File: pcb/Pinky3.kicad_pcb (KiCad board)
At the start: 2 copper layers, 137 x 100.9 mm, 67 parts, among them J1 MJ-4PP-9, P1 i2c-pin, P2 i2c-pin, SW1 RESET_SW, SW10 SW_PUSH, SW11 SW_PUSH, SW12 SW_PUSH, SW13 SW_PUSH, SW14 SW_PUSH, SW15 SW_PUSH, SW16 SW_PUSH, SW17 SW_PUSH, SW18 SW_PUSH, SW19 SW_PUSH, SW2 SW_PUSH, SW20 SW_PUSH, SW21 SW_PUSH, SW22 SW_PUSH, SW23 SW_PUSH, SW24 SW_PUSH, SW25 SW_PUSH, SW26 SW_PUSH, SW3 SW_PUSH, SW4 SW_PUSH, SW5 SW_PUSH, SW6 SW_PUSH, SW7 SW_PUSH, SW8 SW_PUSH, SW9 SW_PUSH, U1 ProMicro

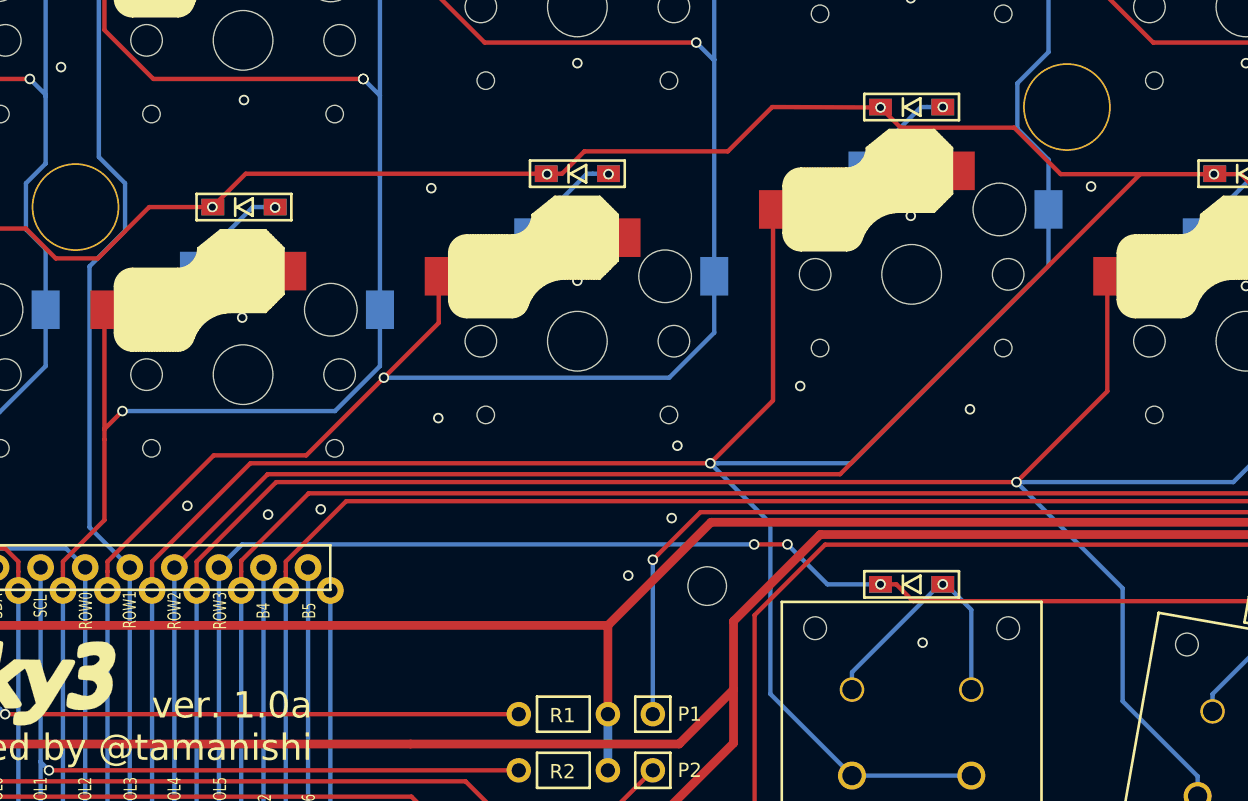
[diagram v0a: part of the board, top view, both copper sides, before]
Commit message: tweak row2
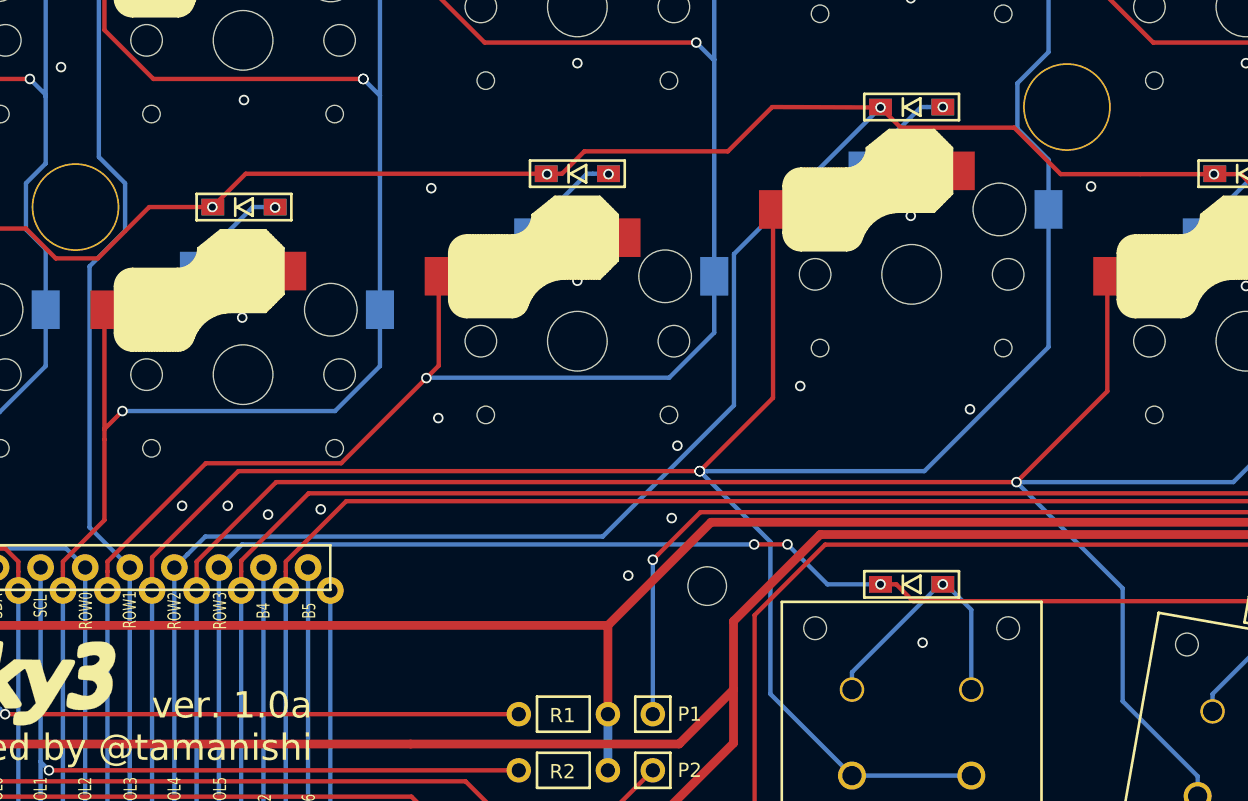
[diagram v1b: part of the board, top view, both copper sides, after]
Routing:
- net row2: track 200.4 -> 192.3 mm
- net col3: track 201.4 -> 204.8 mm, vias 4 -> 5
- net col2: track 145.2 -> 144.2 mm
- net GND: vias 56 -> 57
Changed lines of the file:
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@@
     (thickness 1.6)
     (drawings 29)
-    (tracks 910)
+    (tracks 912)
     (zones 0)
     (modules 67)
@@
   (segment (start 154.85 103.3) (end 156.325 103.3) (width 0.25) (layer F.Cu) (net 7))
   (segment (start 152.32499 100.77499) (end 154.85 103.3) (width 0.25) (layer F.Cu) (net 7))
-  (segment (start 113.876999 102.023001) (end 120.175 95.725) (width 0.25) (layer F.Cu) (net 7))
-  (segment (start 113.875001 102.023001) (end 113.876999 102.023001) (width 0.25) (layer F.Cu) (net 7))
-  (segment (start 103.073012 112.82499) (end 113.875001 102.023001) (width 0.25) (layer F.Cu) (net 7))
-  (segment (start 70.45061 112.82499) (end 103.073012 112.82499) (width 0.25) (layer F.Cu) (net 7))
-  (segment (start 65.132 118.1436) (end 70.45061 112.82499) (width 0.25) (layer F.Cu) (net 7))
   (segment (start 120.175 95.725) (end 115.643998 95.725) (width 0.25) (layer F.Cu) (net 7))
   (segment (start 120.175 95.725) (end 124.375 95.725) (width 0.25) (layer F.Cu) (net 7))
+  (segment (start 66.90061 116.37499) (end 65.893999 117.381601) (width 0.25) (layer B.Cu) (net 7))
+  (segment (start 65.893999 117.381601) (end 65.132 118.1436) (width 0.25) (layer B.Cu) (net 7))
+  (segment (start 89.550012 116.37499) (end 66.90061 116.37499) (width 0.25) (layer B.Cu) (net 7))
+  (segment (start 97.025001 108.900001) (end 89.550012 116.37499) (width 0.25) (layer B.Cu) (net 7))
+  (segment (start 97.025001 100.274999) (end 97.025001 108.900001) (width 0.25) (layer B.Cu) (net 7))
+  (segment (start 105.375 91.925) (end 97.025001 100.274999) (width 0.25) (layer B.Cu) (net 7))
   (segment (start 89.7 74.8) (end 89.875 74.8) (width 0.25) (layer B.Cu) (net 8))
   (segment (start 85.3 70.4) (end 89.7 74.8) (width 0.25) (layer B.Cu) (net 8))
@@
   (via (at 144.575 113.525) (size 0.6) (drill 0.4) (layers F.Cu B.Cu) (net 30))
   (via (at 70.475 115.125) (size 0.6) (drill 0.4) (layers F.Cu B.Cu) (net 30))
-  (via (at 65.875 114.625) (size 0.6) (drill 0.4) (layers F.Cu B.Cu) (net 30))
   (via (at 163.175 111.625) (size 0.6) (drill 0.4) (layers F.Cu B.Cu) (net 30))
+  (via (at 65.575 114.625) (size 0.6) (drill 0.4) (layers F.Cu B.Cu) (net 30))
+  (via (at 68.175 114.625) (size 0.6) (drill 0.4) (layers F.Cu B.Cu) (net 30))
   (segment (start 48.622 133.024838) (end 48.622 134.69) (width 0.25) (layer B.Cu) (net 31) (status 20))
   (segment (start 47.352 131.754838) (end 48.622 133.024838) (width 0.25) (layer B.Cu) (net 31))
@@
   (segment (start 95.85 89.2) (end 95.9 89.2) (width 0.25) (layer B.Cu) (net 38))
   (segment (start 95.9 70.4) (end 95.9 89.2) (width 0.25) (layer B.Cu) (net 38))
-  (segment (start 80.2 101.545) (end 80.2 104.198998) (width 0.25) (layer F.Cu) (net 38))
-  (segment (start 95.9 104.758002) (end 93.333002 107.325) (width 0.25) (layer B.Cu) (net 38))
-  (segment (start 95.9 101.545) (end 95.9 104.758002) (width 0.25) (layer B.Cu) (net 38))
-  (via (at 77.074499 107.324499) (size 0.6) (drill 0.4) (layers F.Cu B.Cu) (net 38))
-  (segment (start 77.075 107.325) (end 77.074499 107.324499) (width 0.25) (layer B.Cu) (net 38))
-  (segment (start 93.333002 107.325) (end 77.075 107.325) (width 0.25) (layer B.Cu) (net 38))
-  (segment (start 80.2 104.198998) (end 77.074499 107.324499) (width 0.25) (layer F.Cu) (net 38))
   (segment (start 61.322 119.45) (end 61.322 132.078) (width 0.25) (layer B.Cu) (net 38))
   (via (at 61.322 132.078) (size 0.6) (drill 0.4) (layers F.Cu B.Cu) (net 38))
   (segment (start 61.322 132.0936) (end 60.052 133.3636) (width 0.25) (layer F.Cu) (net 38))
   (segment (start 61.322 132.078) (end 61.322 132.0936) (width 0.25) (layer F.Cu) (net 38))
-  (segment (start 61.322 117.804838) (end 61.322 118.37237) (width 0.25) (layer F.Cu) (net 38))
   (segment (start 61.322 118.37237) (end 61.322 119.45) (width 0.25) (layer F.Cu) (net 38))
-  (segment (start 67.376858 111.74998) (end 61.322 117.804838) (width 0.25) (layer F.Cu) (net 38))
-  (segment (start 72.649018 111.74998) (end 67.376858 111.74998) (width 0.25) (layer F.Cu) (net 38))
-  (segment (start 77.074499 107.324499) (end 72.649018 111.74998) (width 0.25) (layer F.Cu) (net 38))
+  (segment (start 66.926848 112.19999) (end 61.322 117.804838) (width 0.25) (layer F.Cu) (net 38))
+  (segment (start 61.322 117.804838) (end 61.322 118.37237) (width 0.25) (layer F.Cu) (net 38))
+  (segment (start 74.641012 112.19999) (end 66.926848 112.19999) (width 0.25) (layer F.Cu) (net 38))
+  (segment (start 80.2 101.545) (end 80.2 106.641002) (width 0.25) (layer F.Cu) (net 38))
+  (segment (start 95.9 104.758002) (end 93.333002 107.325) (width 0.25) (layer B.Cu) (net 38))
+  (segment (start 95.9 101.545) (end 95.9 104.758002) (width 0.25) (layer B.Cu) (net 38))
+  (segment (start 79.516002 107.325) (end 79.495501 107.345501) (width 0.25) (layer B.Cu) (net 38))
+  (segment (start 93.333002 107.325) (end 79.516002 107.325) (width 0.25) (layer B.Cu) (net 38))
+  (segment (start 79.495501 107.345501) (end 74.641012 112.19999) (width 0.25) (layer F.Cu) (net 38))
+  (via (at 79.495501 107.345501) (size 0.6) (drill 0.4) (layers F.Cu B.Cu) (net 38))
+  (segment (start 80.2 106.641002) (end 79.495501 107.345501) (width 0.25) (layer F.Cu) (net 38))
   (segment (start 63.862 119.45) (end 63.862 132.072) (width 0.25) (layer B.Cu) (net 39) (status 10))
   (via (at 63.862 132.072) (size 0.6) (drill 0.4) (layers F.Cu B.Cu) (net 39))
@@
   (segment (start 110.549844 130) (end 110.550008 130.000164) (width 0.25) (layer B.Cu) (net 39))
   (segment (start 103.75 130) (end 110.549844 130) (width 0.25) (layer B.Cu) (net 39))
-  (via (at 95.675 112.19999) (size 0.6) (drill 0.4) (layers F.Cu B.Cu) (net 39))
-  (segment (start 99.25 108.62499) (end 95.675 112.19999) (width 0.25) (layer F.Cu) (net 39))
-  (segment (start 99.25 97.735) (end 99.25 108.62499) (width 0.25) (layer F.Cu) (net 39))
-  (segment (start 99.100001 115.624991) (end 95.675 112.19999) (width 0.25) (layer B.Cu) (net 39))
-  (segment (start 99.100001 125.350001) (end 99.100001 115.624991) (width 0.25) (layer B.Cu) (net 39))
   (segment (start 103.75 130) (end 99.100001 125.350001) (width 0.25) (layer B.Cu) (net 39))
-  (segment (start 63.862 117.804838) (end 63.862 118.37237) (width 0.25) (layer F.Cu) (net 39))
-  (segment (start 69.466848 112.19999) (end 63.862 117.804838) (width 0.25) (layer F.Cu) (net 39))
-  (segment (start 63.862 118.37237) (end 63.862 119.45) (width 0.25) (layer F.Cu) (net 39))
-  (segment (start 95.675 112.19999) (end 69.466848 112.19999) (width 0.25) (layer F.Cu) (net 39))
-  (segment (start 96.099264 112.19999) (end 95.675 112.19999) (width 0.25) (layer B.Cu) (net 39))
-  (segment (start 114.95 100.948002) (end 103.698012 112.19999) (width 0.25) (layer B.Cu) (net 39))
-  (segment (start 103.698012 112.19999) (end 96.099264 112.19999) (width 0.25) (layer B.Cu) (net 39))
-  (segment (start 114.95 97.735) (end 114.95 100.948002) (width 0.25) (layer B.Cu) (net 39))
+  (via (at 95.075 112.65) (size 0.6) (drill 0.4) (layers F.Cu B.Cu) (net 39))
+  (segment (start 99.25 108.475) (end 95.075 112.65) (width 0.25) (layer F.Cu) (net 39))
+  (segment (start 99.25 97.735) (end 99.25 108.475) (width 0.25) (layer F.Cu) (net 39))
+  (segment (start 99.100001 116.675001) (end 95.075 112.65) (width 0.25) (layer B.Cu) (net 39))
+  (segment (start 99.100001 125.350001) (end 99.100001 116.675001) (width 0.25) (layer B.Cu) (net 39))
+  (segment (start 107.875002 112.65) (end 95.499264 112.65) (width 0.25) (layer B.Cu) (net 39))
+  (segment (start 114.95 105.575002) (end 107.875002 112.65) (width 0.25) (layer B.Cu) (net 39))
+  (segment (start 95.499264 112.65) (end 95.075 112.65) (width 0.25) (layer B.Cu) (net 39))
+  (segment (start 114.95 97.735) (end 114.95 105.575002) (width 0.25) (layer B.Cu) (net 39))
+  (via (at 95.075 112.65) (size 0.6) (drill 0.4) (layers F.Cu B.Cu) (net 39))
+  (segment (start 63.862 117.563002) (end 63.862 119.45) (width 0.25) (layer F.Cu) (net 39))
+  (segment (start 68.775002 112.65) (end 63.862 117.563002) (width 0.25) (layer F.Cu) (net 39))
+  (segment (start 95.075 112.65) (end 68.775002 112.65) (width 0.25) (layer F.Cu) (net 39))
   (segment (start 134 63.445) (end 134 64.795) (width 0.25) (layer B.Cu) (net 40))
   (segment (start 134 82.495) (end 134 83.845) (width 0.25) (layer B.Cu) (net 40))
